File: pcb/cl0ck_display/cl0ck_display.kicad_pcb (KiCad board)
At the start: 2 copper layers, 307 x 27 mm, 16 parts, among them P1 CONN_01X03, P2 CONN_01X02

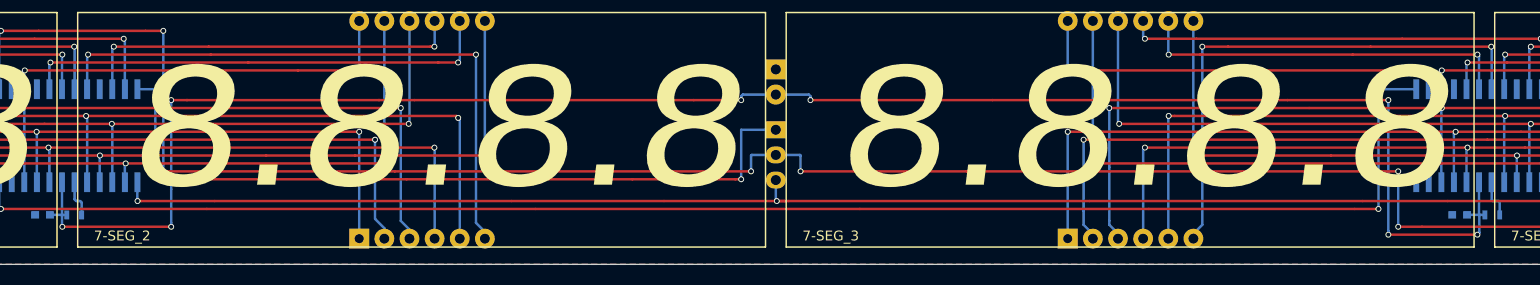
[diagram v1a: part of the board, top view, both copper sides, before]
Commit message: Revision to pcbs.
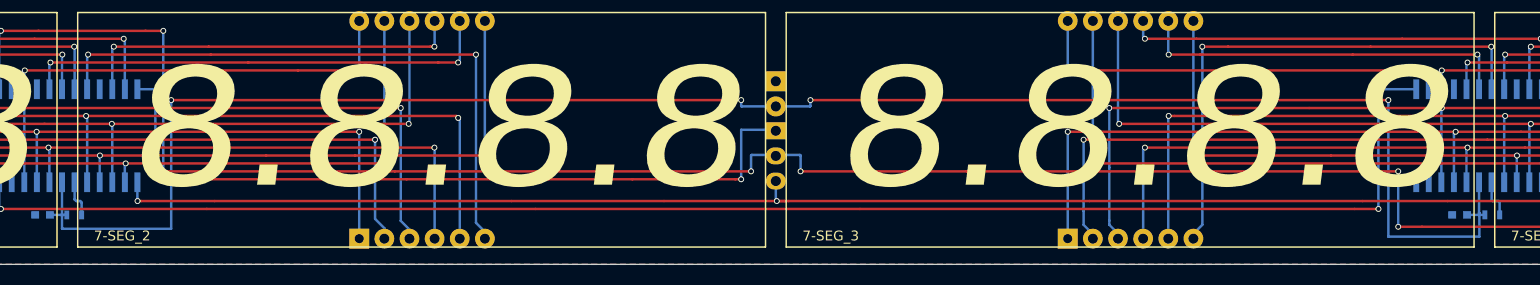
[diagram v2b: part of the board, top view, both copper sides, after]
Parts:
- moved P2 1.20 mm to (203.5, 135.5)
- moved P1 0.10 mm to (203.5, 140.5)
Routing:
- net VCC: track 183.8 -> 185.2 mm, vias 8 -> 4
